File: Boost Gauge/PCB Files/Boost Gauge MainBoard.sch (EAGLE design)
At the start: 76 parts, among them IC1 MCT6SD, IC2 MCP96RL00-E_MX, IC4 ATMEGA328PB-AN, IC6 7805DT, IC7 MCP25625-E_SS, Q1 BUK7Y6R0-60EX

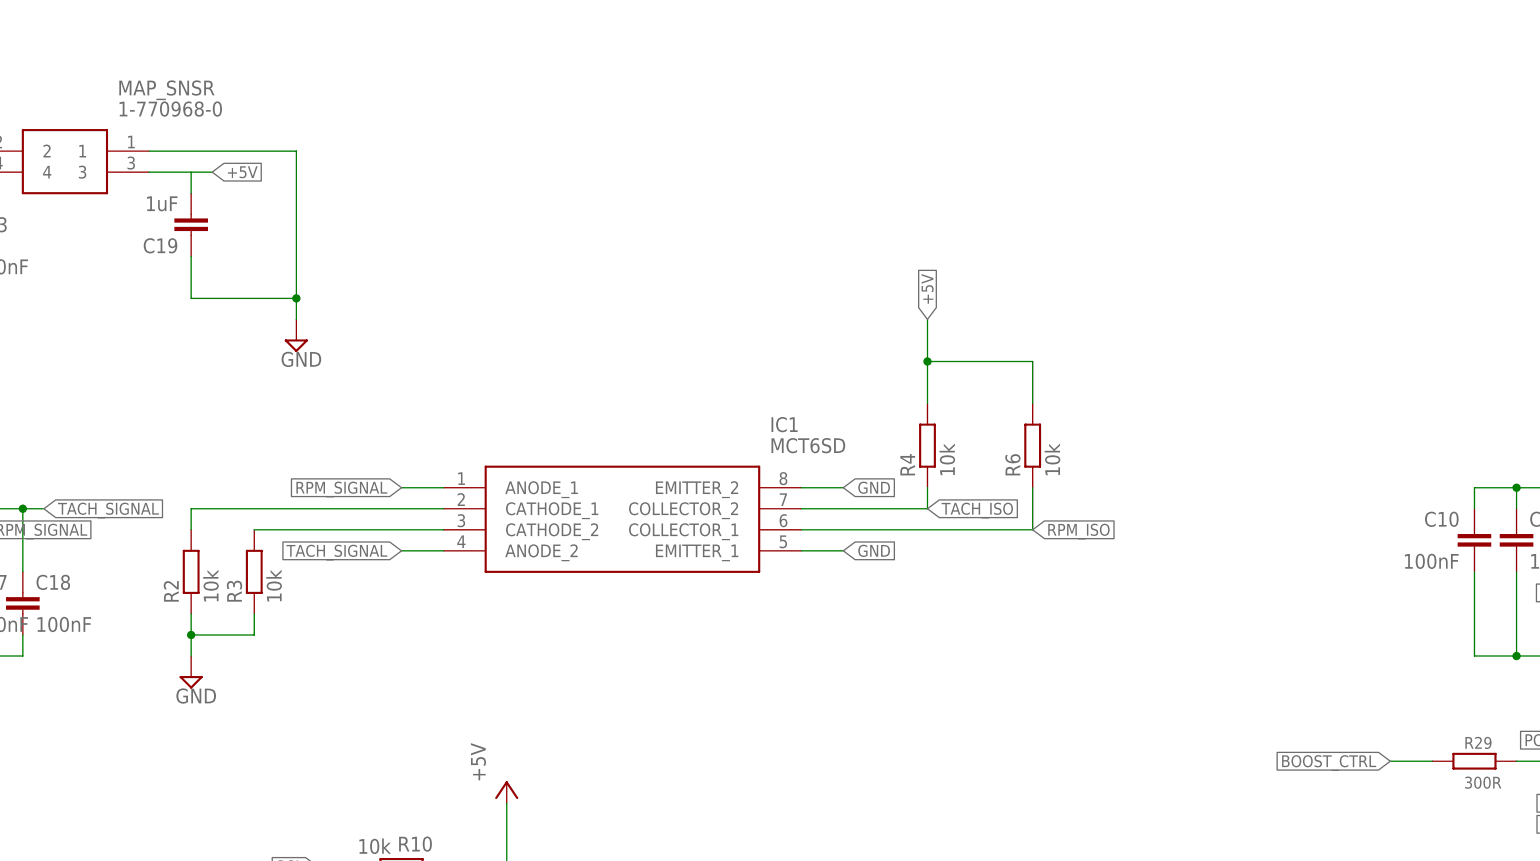
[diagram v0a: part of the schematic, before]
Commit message: v0.2 PCB
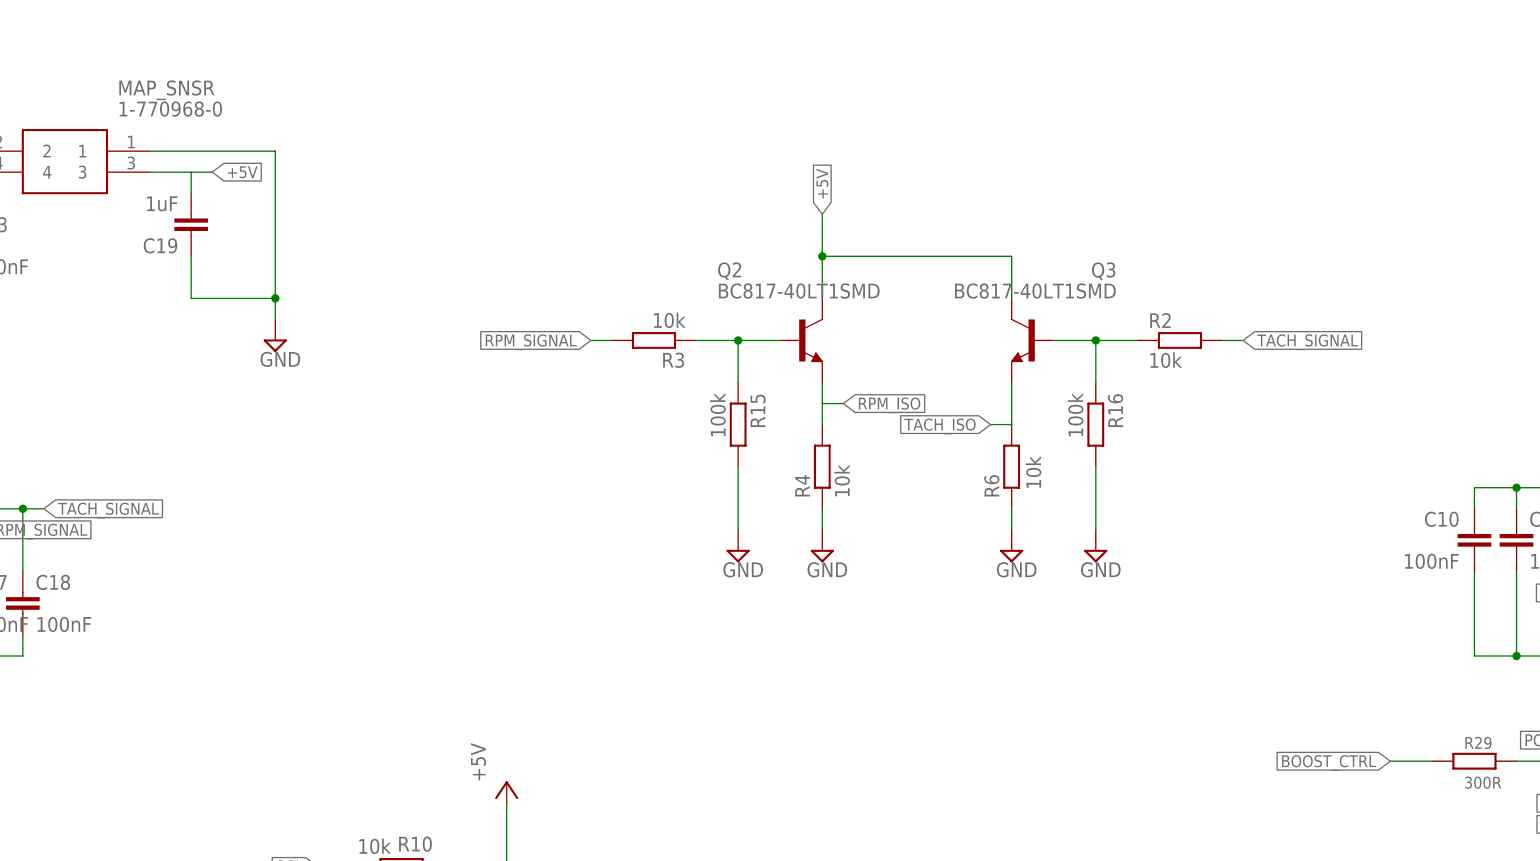
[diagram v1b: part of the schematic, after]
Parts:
- removed IC1: MCT6SD, MCT6SD:MCT6SD
- added Q2, Q3: BC817-40LT1SMD, transistor-npn:BC817-40LT1SMD
- added R15, R16: 100k, rcl:R-EU_R0805
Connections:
- removed net N$2: IC1.CATHODE_1, R2.2
- new net N$4: Q3.B, R16.1, R2.1
- net +5V: now also Q2.C, Q3.C; no longer R4.2, R6.2
- net GND: now also R15.2, R16.2, R4.1, R6.1; no longer IC1.EMITTER_1, IC1.EMITTER_2, R2.1, R3.1
- net N$3: now also Q2.B, R15.1, R3.1; no longer IC1.CATHODE_2, R3.2
- net RPM_ISO: now also Q2.E, R4.2; no longer IC1.COLLECTOR_1, R6.1
- net RPM_SIGNAL: now also R3.2; no longer IC1.ANODE_1
- net TACH_ISO: now also Q3.E, R6.2; no longer IC1.COLLECTOR_2, R4.1
- net TACH_SIGNAL: now also R2.2; no longer IC1.ANODE_2
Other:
- moved on the sheet: R2, R3, R4, R6

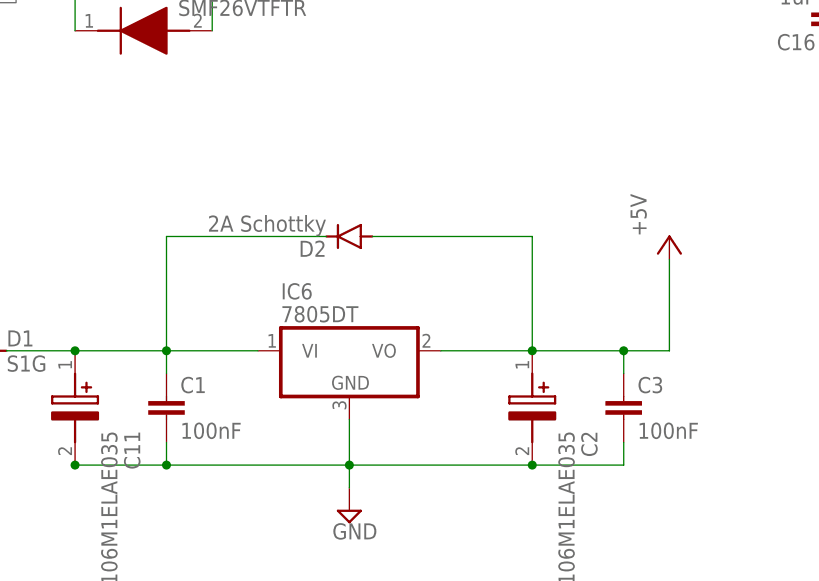
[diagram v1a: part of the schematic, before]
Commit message: V1.0 of the mainboard files
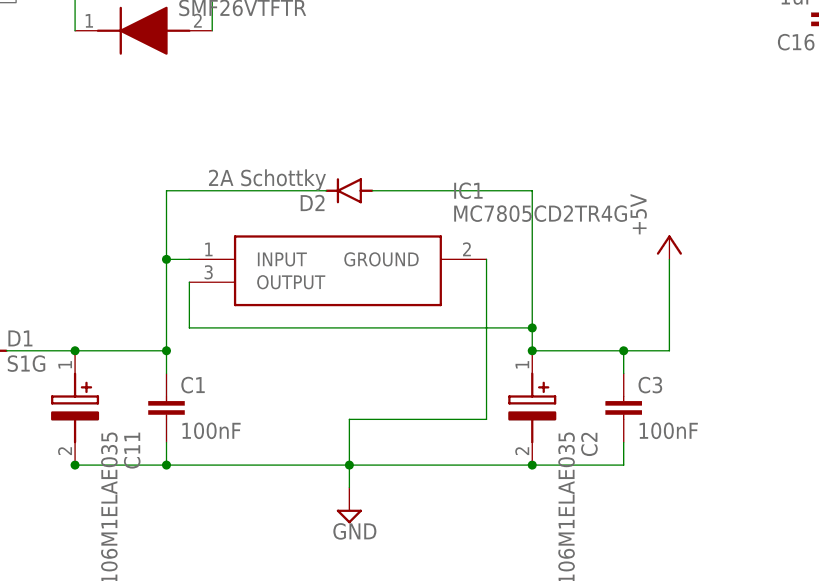
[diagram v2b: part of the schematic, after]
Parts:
- removed IC6: 7805DT, linear:7805DT
- added IC1: MC7805CD2TR4G, MC7805CD2TR4G:MC7805CD2TR4G
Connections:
- net +5V: now also IC1.OUTPUT; no longer IC6.VO
- net GND: now also IC1.GROUND; no longer IC6.GND
- net N$6: now also IC1.INPUT; no longer IC6.VI
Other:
- moved on the sheet: D2
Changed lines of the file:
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@@
 <parts>
 <part name="Q1" library="BUK7Y6R0-60EX" deviceset="BUK7Y6R0-60EX" device=""/>
-<part name="IC6" library="linear" library_urn="urn:adsk.eagle:library:262" deviceset="78*" device="DT" package3d_urn="urn:adsk.eagle:package:16415/2" technology="05"/>
 <part name="C1" library="rcl" library_urn="urn:adsk.eagle:library:334" deviceset="C-EU" device="C0805" package3d_urn="urn:adsk.eagle:package:23617/2" value="100nF"/>
 <part name="D1" library="diode" library_urn="urn:adsk.eagle:library:210" deviceset="DIODE-" device="DO-214AC" package3d_urn="urn:adsk.eagle:package:43416/2" value="S1G"/>
@@
 <part name="SUPPLY3" library="supply2" library_urn="urn:adsk.eagle:library:372" deviceset="GND" device=""/>
 <part name="SUPPLY20" library="supply2" library_urn="urn:adsk.eagle:library:372" deviceset="GND" device=""/>
+<part name="IC1" library="MC7805CD2TR4G" deviceset="MC7805CD2TR4G" device=""/>
 </parts>
 <sheets>
@@
 <attribute name="VALUE" x="-62.23" y="139.7" size="1.778" layer="96" rot="R180" align="center-left"/>
 </instance>
-<instance part="IC6" gate="A1" x="40.64" y="147.32" smashed="yes">
-<attribute name="NAME" x="33.02" y="153.035" size="1.778" layer="95"/>
-<attribute name="VALUE" x="33.02" y="150.495" size="1.778" layer="96"/>
-</instance>
 <instance part="C1" gate="G$1" x="20.32" y="142.24" smashed="yes">
 <attribute name="NAME" x="21.844" y="142.621" size="1.778" layer="95"/>
@@
 <attribute name="VALUE" x="-93.345" y="123.825" size="1.778" layer="96"/>
 </instance>
-<instance part="D2" gate="G$1" x="40.64" y="160.02" smashed="yes" rot="R180">
-<attribute name="NAME" x="38.1" y="159.5374" size="1.778" layer="95" rot="R180"/>
-<attribute name="VALUE" x="38.1" y="162.3314" size="1.778" layer="96" rot="R180"/>
+<instance part="D2" gate="G$1" x="40.64" y="165.1" smashed="yes" rot="R180">
+<attribute name="NAME" x="38.1" y="164.6174" size="1.778" layer="95" rot="R180"/>
+<attribute name="VALUE" x="38.1" y="167.4114" size="1.778" layer="96" rot="R180"/>
 </instance>
 <instance part="IC4" gate="G$1" x="15.24" y="35.56" smashed="yes">
@@
 <instance part="SUPPLY20" gate="GND" x="-124.46" y="53.34" smashed="yes">
 <attribute name="VALUE" x="-126.365" y="50.165" size="1.778" layer="96"/>
+</instance>
+<instance part="IC1" gate="G$1" x="22.86" y="157.48" smashed="yes">
+<attribute name="NAME" x="52.07" y="165.1" size="1.778" layer="95" align="center-left"/>
+<attribute name="VALUE" x="52.07" y="162.56" size="1.778" layer="96" align="center-left"/>
 </instance>
 </instances>
@@
 <pinref part="SUPPLY1" gate="GND" pin="GND"/>
 <wire x1="40.64" y1="132.08" x2="40.64" y2="134.62" width="0.1524" layer="91"/>
-<pinref part="IC6" gate="A1" pin="GND"/>
 <pinref part="C1" gate="G$1" pin="2"/>
 <wire x1="40.64" y1="134.62" x2="40.64" y2="139.7" width="0.1524" layer="91"/>
@@
 <wire x1="60.96" y1="134.62" x2="40.64" y2="134.62" width="0.1524" layer="91"/>
 <junction x="60.96" y="134.62"/>
+<pinref part="IC1" gate="G$1" pin="GROUND"/>
+<wire x1="55.88" y1="157.48" x2="55.88" y2="139.7" width="0.1524" layer="91"/>
+<wire x1="55.88" y1="139.7" x2="40.64" y2="139.7" width="0.1524" layer="91"/>
 </segment>
 <segment>
@@
 </segment>
 <segment>
-<pinref part="IC6" gate="A1" pin="VO"/>
-<wire x1="50.8" y1="147.32" x2="60.96" y2="147.32" width="0.1524" layer="91"/>
 <pinref part="P+2" gate="1" pin="+5V"/>
 <wire x1="60.96" y1="147.32" x2="71.12" y2="147.32" width="0.1524" layer="91"/>
@@
 <junction x="71.12" y="147.32"/>
 <pinref part="D2" gate="G$1" pin="A"/>
-<wire x1="43.18" y1="160.02" x2="60.96" y2="160.02" width="0.1524" layer="91"/>
-<wire x1="60.96" y1="160.02" x2="60.96" y2="147.32" width="0.1524" layer="91"/>
+<wire x1="43.18" y1="165.1" x2="60.96" y2="165.1" width="0.1524" layer="91"/>
+<wire x1="60.96" y1="165.1" x2="60.96" y2="149.86" width="0.1524" layer="91"/>
 <pinref part="C2" gate="G$1" pin="+"/>
+<pinref part="IC1" gate="G$1" pin="OUTPUT"/>
+<wire x1="60.96" y1="149.86" x2="60.96" y2="147.32" width="0.1524" layer="91"/>
+<wire x1="22.86" y1="154.94" x2="22.86" y2="149.86" width="0.1524" layer="91"/>
+<wire x1="22.86" y1="149.86" x2="60.96" y2="149.86" width="0.1524" layer="91"/>
+<junction x="60.96" y="149.86"/>
 </segment>
 <segment>
@@
 <segment>
 <pinref part="D1" gate="G$1" pin="C"/>
-<pinref part="IC6" gate="A1" pin="VI"/>
 <wire x1="2.54" y1="147.32" x2="10.16" y2="147.32" width="0.1524" layer="91"/>
 <pinref part="D2" gate="G$1" pin="C"/>
 <wire x1="10.16" y1="147.32" x2="20.32" y2="147.32" width="0.1524" layer="91"/>
-<wire x1="20.32" y1="147.32" x2="30.48" y2="147.32" width="0.1524" layer="91"/>
-<wire x1="38.1" y1="160.02" x2="20.32" y2="160.02" width="0.1524" layer="91"/>
-<wire x1="20.32" y1="160.02" x2="20.32" y2="147.32" width="0.1524" layer="91"/>
+<wire x1="38.1" y1="165.1" x2="20.32" y2="165.1" width="0.1524" layer="91"/>
+<wire x1="20.32" y1="165.1" x2="20.32" y2="157.48" width="0.1524" layer="91"/>
 <junction x="20.32" y="147.32"/>
 <pinref part="C1" gate="G$1" pin="1"/>
+<wire x1="20.32" y1="157.48" x2="20.32" y2="147.32" width="0.1524" layer="91"/>
 <wire x1="20.32" y1="147.32" x2="20.32" y2="144.78" width="0.1524" layer="91"/>
 <pinref part="C11" gate="G$1" pin="+"/>
 <junction x="10.16" y="147.32"/>
-</segment>
-</net>
+<pinref part="IC1" gate="G$1" pin="INPUT"/>
+<wire x1="22.86" y1="157.48" x2="20.32" y2="157.48" width="0.1524" layer="91"/>
+<junction x="20.32" y="157.48"/>
+</segment>
+</net>
